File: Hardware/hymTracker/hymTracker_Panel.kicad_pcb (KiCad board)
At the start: 2 copper layers, 93 x 96.1 mm, 38 parts, among them J1 DB9_Female, Q1 2N7000, U1 MP1584_DCDC, U2 GY-NEO6MV2

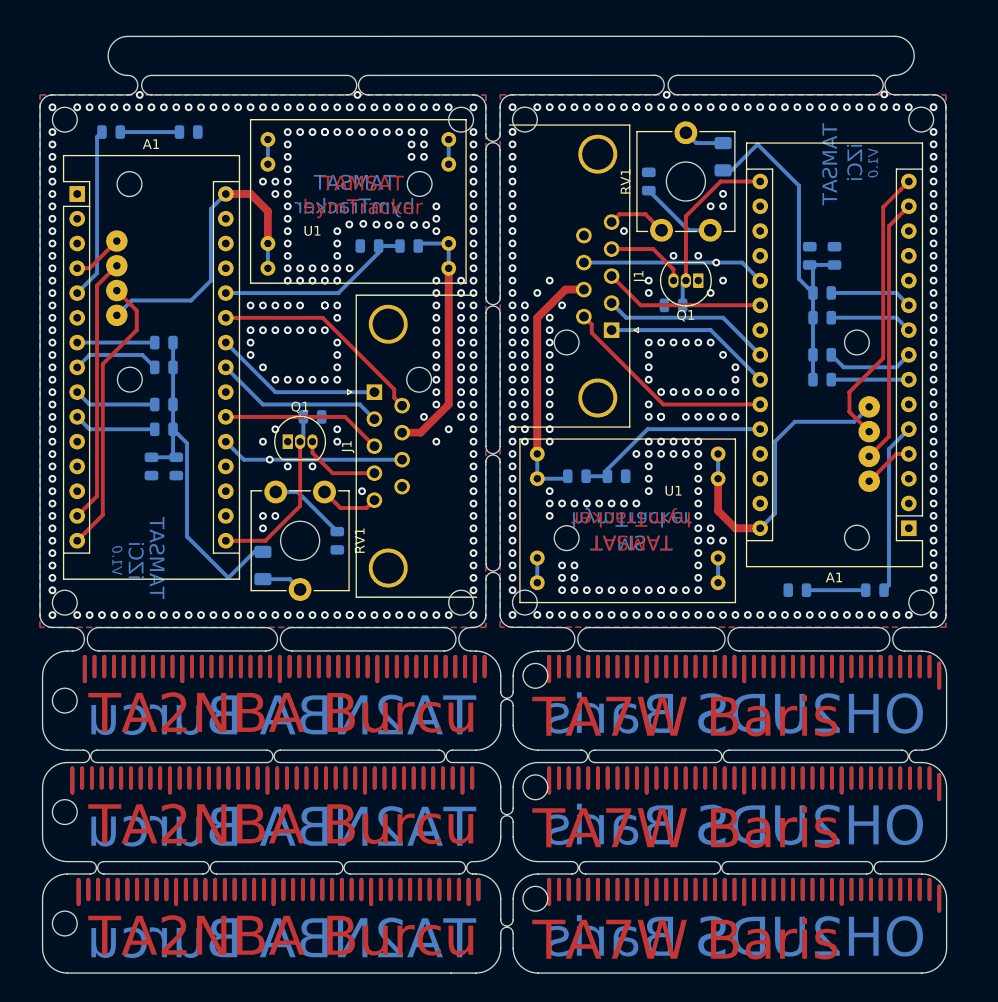
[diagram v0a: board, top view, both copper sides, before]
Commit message: re-branding
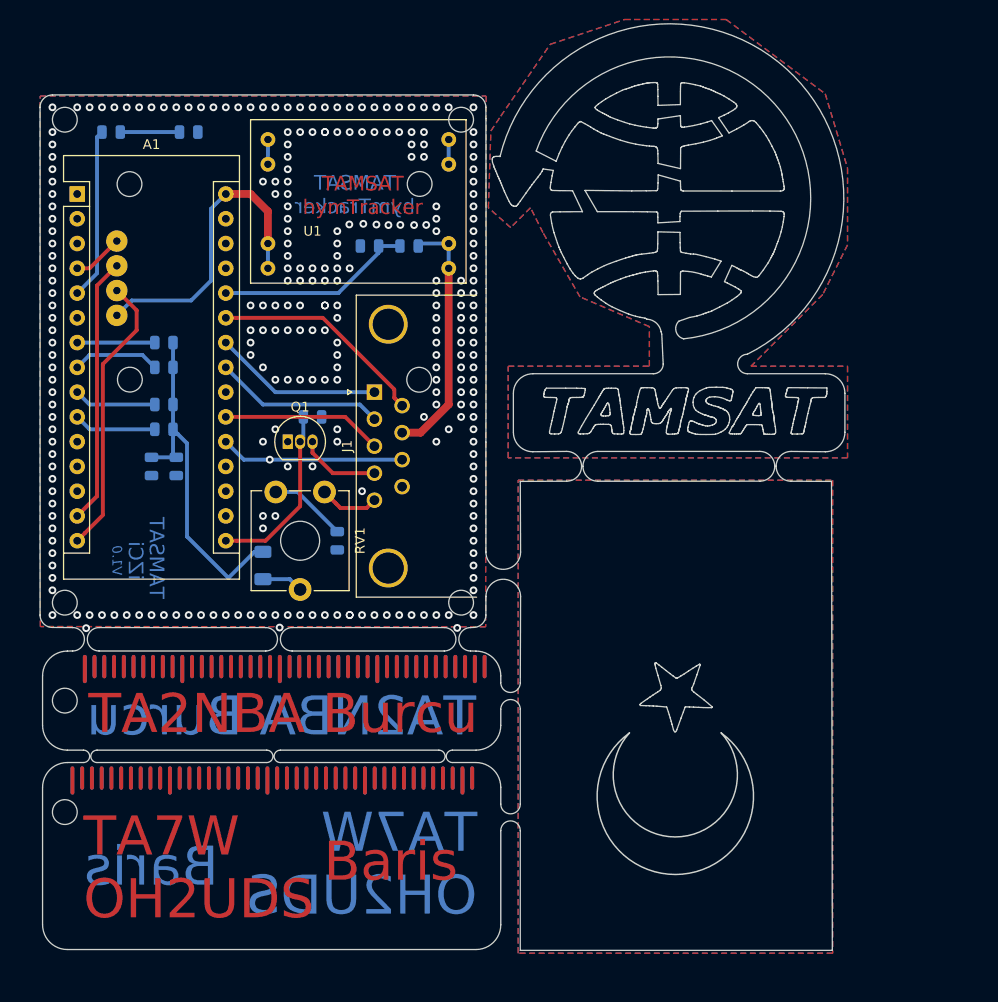
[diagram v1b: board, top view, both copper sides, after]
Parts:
- removed the A1 at (118.0, 92.8)
- removed the C1 at (110.4, 64.9)
- removed the C2 at (99.0, 54.7)
- removed the D1 at (106.6, 99.2)
- removed the J1 at (87.6, 72.5)
- removed the Q1 at (96.5, 67.4)
- removed the R1 at (84.0, 87.5)
- removed the R10 at (91.4, 57.3)
- removed the R2 at (88.1, 87.5)
- removed the R3 at (114.6, 99.2)
- removed the R4 at (109.2, 77.6)
- removed the R5 at (109.2, 75.0)
- removed the R6 at (109.2, 71.2)
- removed the R7 at (109.2, 68.7)
- removed the R8 at (93.9, 70.0)
- removed the R9 at (107.9, 64.9)
- removed the RV1 at (97.7, 62.3)
- removed the U1 at (87.6, 90.3)
- removed the U2 at (97.7, 82.7)
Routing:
- net (no net): track 1402.3 -> 346.0 mm, vias 279 -> 0
- net GND: vias 248 -> 262
- net /PTT: vias 0 -> 2
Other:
- board size 93 x 96.1 mm -> 82.5 x 95 mm
- board text added: "Baris"
- board text added: "TA7W OH2UDS"
- board text removed: "OH2UDS Baris"
- board text removed: "TA7W Baris"
